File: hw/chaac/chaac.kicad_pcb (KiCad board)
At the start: 2 copper layers, 42 x 55 mm, 56 parts, among them J1 Battery, J2 TC2030-CTX, J3 UART, J4 windrain, Q1 Q_PMOS_GSD, SW1 RST, SW2 RST, U1 TPS7A0530PDBVT, U2 NRF52811-QFAA, U3 BMP280, U4 SHT3x-DIS, U5 E22-X00M22S, Y2 32.768kHz

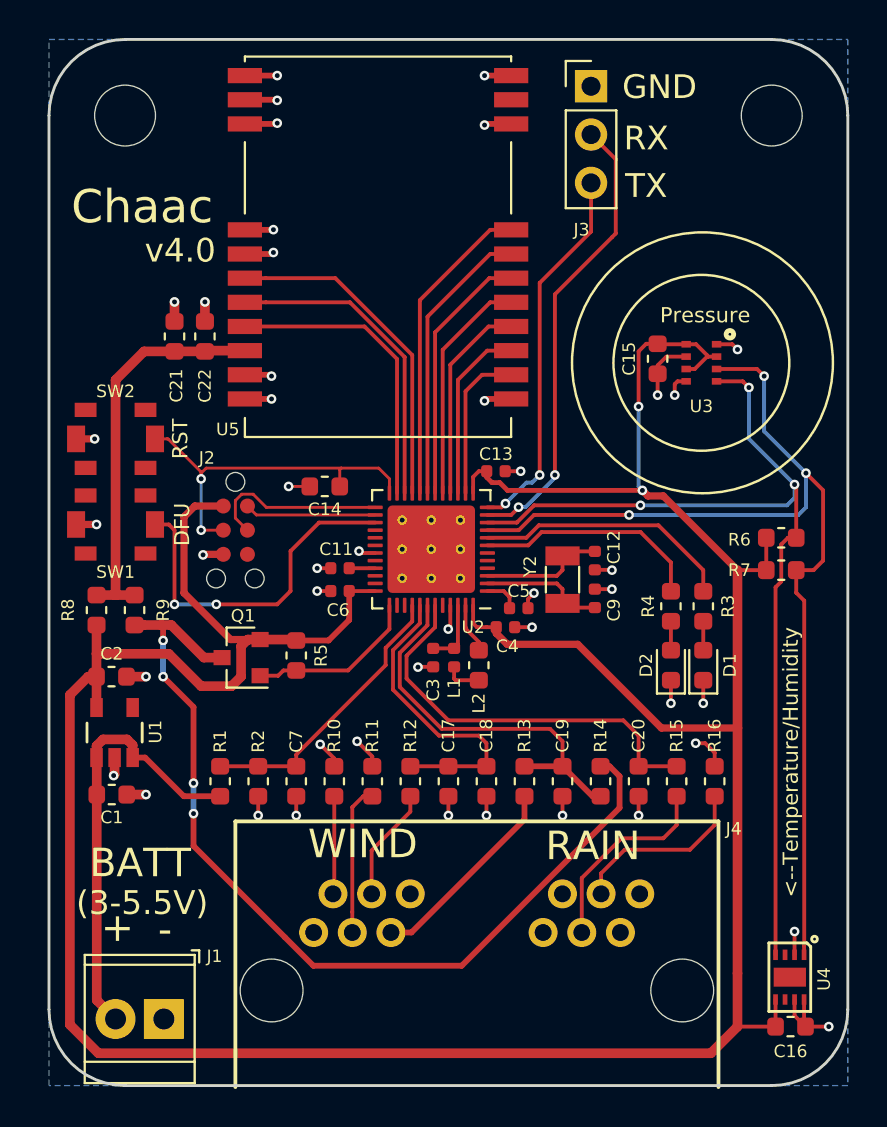
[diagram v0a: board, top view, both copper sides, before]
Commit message: Adding chaac v5.0
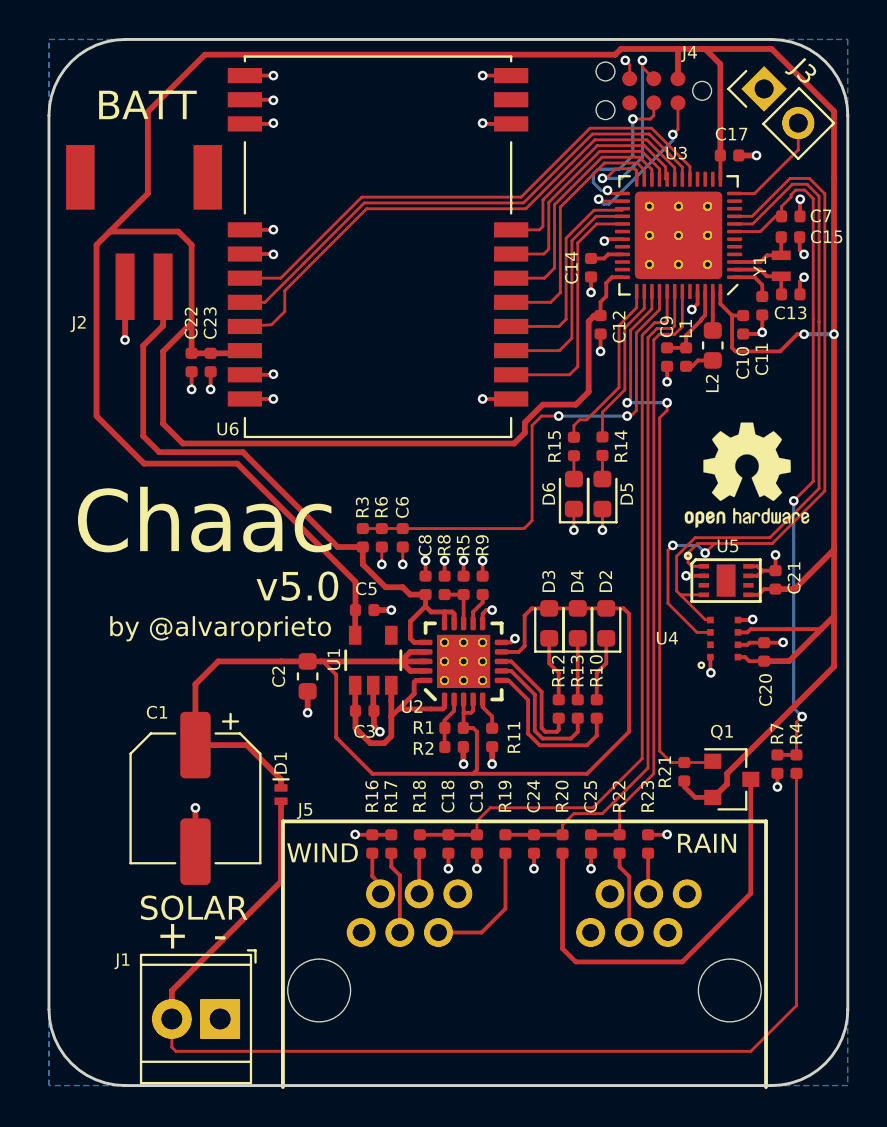
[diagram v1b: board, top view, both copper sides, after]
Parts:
- removed the C14 at (117.5, 152.5)
- removed C16: 0.1uF, Capacitor_SMD:C_0603_1608Metric
- removed the R14 at (132.0, 168.0)
- removed the REF** at (124.4, 151.0)
- removed the REF** at (141.0, 133.0)
- removed the REF** at (107.0, 133.0)
- removed SW1, SW2: RST, alvarop:PTS820J25MSMTRLFS
- removed the U3 at (137.3, 146.0)
- added C2: 10uF, Resistor_SMD:R_0603_1608Metric, F.Cu at (116.6, 162.5)
- added C21: 0.1uF, Capacitor_SMD:C_0402_1005Metric, F.Cu at (141.2, 157.4)
- added C3: 4.7uF, Capacitor_SMD:C_0402_1005Metric, F.Cu at (119.6, 164.3)
- added C7: 0.1uF, Capacitor_SMD:C_0402_1005Metric, F.Cu at (142.0, 138.3)
- added C8: 4.7uF, Capacitor_SMD:C_0402_1005Metric, F.Cu at (122.8, 157.7)
- added D1: RB521CS30L,315, alvarop:RB521CS30L, F.Cu at (115.2, 168.7)
- added D2: LED_ALT, LED_SMD:LED_0603_1608Metric, F.Cu at (132.3, 159.7)
- added D3: LED_ALT, LED_SMD:LED_0603_1608Metric, F.Cu at (129.3, 159.7)
- added D4: LED_ALT, LED_SMD:LED_0603_1608Metric, F.Cu at (130.8, 159.7)
- added G***: LOGO, alvarop:weather_station, B.Cu at (115.0, 156.0)
- added J2: Battery, alvarop:S2B-PH-SM4-TB, F.Cu at (108.0, 142.0)
- added R1: 270k, Resistor_SMD:R_0402_1005Metric, F.Cu at (124.3, 165.2)
- added R10: 10k, Resistor_SMD:R_0402_1005Metric, F.Cu at (131.8, 164.2)
- added R11: 10k, Resistor_SMD:R_0402_1005Metric, F.Cu at (126.3, 165.7)
- added R12: 10k, Resistor_SMD:R_0402_1005Metric, F.Cu at (129.8, 164.2)
- added R13: 10k, Resistor_SMD:R_0402_1005Metric, F.Cu at (130.8, 164.2)
- added R20: 10k, Resistor_SMD:R_0402_1005Metric, F.Cu at (130.0, 171.3)
- added R4: 1M, Resistor_SMD:R_0402_1005Metric, F.Cu at (142.3, 167.1)
- added R5: 100k, Resistor_SMD:R_0402_1005Metric, F.Cu at (124.8, 157.7)
- added REF**: OSHW-Logo2_7.3x6mm_SilkScreen, Symbol:OSHW-Logo2_7.3x6mm_SilkScreen, F.Cu at (139.7, 151.9)
- added U2: MCP73871, alvarop:MCP73871, F.Cu at (124.8, 161.7)
- added U5: SHT3x-DIS, alvarop:SHT3x, F.Cu at (138.6, 157.4)
- C1: value 1uF -> 100uF; footprint Capacitor_SMD:C_0603_1608Metric -> Capacitor_SMD:CP_Elec_6.3x5.4
- C18: renamed from C17; footprint Capacitor_SMD:C_0603_1608Metric -> Capacitor_SMD:C_0402_1005Metric
- C19: renamed from C18; footprint Capacitor_SMD:C_0603_1608Metric -> Capacitor_SMD:C_0402_1005Metric
- C20: renamed from C15; footprint Capacitor_SMD:C_0603_1608Metric -> Capacitor_SMD:C_0402_1005Metric
- C22: renamed from C21; footprint Capacitor_SMD:C_0603_1608Metric -> Capacitor_SMD:C_0402_1005Metric
- C23: renamed from C22; footprint Capacitor_SMD:C_0603_1608Metric -> Capacitor_SMD:C_0402_1005Metric
- C24: renamed from C19; footprint Capacitor_SMD:C_0603_1608Metric -> Capacitor_SMD:C_0402_1005Metric
- C25: renamed from C20; footprint Capacitor_SMD:C_0603_1608Metric -> Capacitor_SMD:C_0402_1005Metric
- C5: renamed from C2; footprint Capacitor_SMD:C_0603_1608Metric -> Capacitor_SMD:C_0402_1005Metric
- C6: renamed from C7; footprint Capacitor_SMD:C_0603_1608Metric -> Capacitor_SMD:C_0402_1005Metric
- J1: value Battery -> Solar
- J3: footprint Connector_PinHeader_2.54mm:PinHeader_1x03_P2.54mm_Vertical -> Connector_PinHeader_2.54mm:PinHeader_1x02_P2.54mm_Vertical
- R14: renamed from R3; footprint Resistor_SMD:R_0603_1608Metric -> Resistor_SMD:R_0402_1005Metric
- R15: renamed from R4; footprint Resistor_SMD:R_0603_1608Metric -> Resistor_SMD:R_0402_1005Metric
- R16: renamed from R10; value 1k -> 0; footprint Resistor_SMD:R_0603_1608Metric -> Resistor_SMD:R_0402_1005Metric
- R17: renamed from R11; footprint Resistor_SMD:R_0603_1608Metric -> Resistor_SMD:R_0402_1005Metric
- R18: renamed from R12; footprint Resistor_SMD:R_0603_1608Metric -> Resistor_SMD:R_0402_1005Metric
- R19: renamed from R13; footprint Resistor_SMD:R_0603_1608Metric -> Resistor_SMD:R_0402_1005Metric
- R2: footprint Resistor_SMD:R_0603_1608Metric -> Resistor_SMD:R_0402_1005Metric
- R21: renamed from R5; footprint Resistor_SMD:R_0603_1608Metric -> Resistor_SMD:R_0402_1005Metric
- R22: renamed from R15; footprint Resistor_SMD:R_0603_1608Metric -> Resistor_SMD:R_0402_1005Metric
- R23: renamed from R16; footprint Resistor_SMD:R_0603_1608Metric -> Resistor_SMD:R_0402_1005Metric
- R3: renamed from R1; value 100k -> 1M; footprint Resistor_SMD:R_0603_1608Metric -> Resistor_SMD:R_0402_1005Metric
- R6, R7: value 4.7k -> 1M; footprint Resistor_SMD:R_0603_1608Metric -> Resistor_SMD:R_0402_1005Metric
- R8: value 0 -> 100k; footprint Resistor_SMD:R_0603_1608Metric -> Resistor_SMD:R_0402_1005Metric
- R9: value 0 -> 1M; footprint Resistor_SMD:R_0603_1608Metric -> Resistor_SMD:R_0402_1005Metric
- U4: value SHT3x-DIS -> DPS368; footprint alvarop:SHT3x -> alvarop:DPS368
- Y1: renamed from Y2; footprint Crystal:Crystal_SMD_3215-2Pin_3.2x1.5mm -> alvarop:ABS05
- moved J4 31.9 mm to (134.8, 131.7), turned to 180 degrees
- moved Q1 26.6 mm to (138.9, 167.9), turned to 0 degrees
- moved R21 21.3 mm to (136.4, 167.5), turned to 270 degrees
- moved U3 21.0 mm to (136.1, 139.3)
- moved R6 21.0 mm to (120.5, 155.2), turned to 90 degrees
- moved L2 20.8 mm to (137.9, 145.1)
- moved C17 20.7 mm to (138.8, 135.1)
- moved C14 20.6 mm to (131.5, 141.0), turned to 270 degrees
- moved C11 20.4 mm to (140.5, 143.0), turned to 90 degrees
- moved C10 20.2 mm to (139.5, 144.0), turned to 90 degrees
- moved Y1 20.1 mm to (141.5, 140.9), turned to 90 degrees
- moved C9 20.0 mm to (135.5, 145.7)
- moved L1 20.0 mm to (136.5, 145.7)
- moved C15 19.9 mm to (142.0, 139.4), turned to 0 degrees
- moved C12 19.6 mm to (132.0, 144.0), turned to 90 degrees
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- renumbered C4 to C10, C5 to C11, C6 to C12, C9 to C13, C11 to C14, C12 to C15, C13 to C17, C3 to C9, D1 to D5, D2 to D6, J2 to J4, J4 to J5, U2 to U3, U5 to U6
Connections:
- C1 pad 1: /VBATT -> /MCP_VIN
- C22 pad 1: Net-(C21-Pad1) -> +3V3
- C23 pad 1: Net-(C21-Pad1) -> +3V3
- J1 pad 2: /VBATT -> /SOLAR_IN
- J3 pad 2: /UART_RX -> /UART_TX
- R2 pad 1: GND -> Net-(R1-Pad2)
- R2 pad 2: /BATT -> GND
- R6 pad 1: /SCL -> GND
- R6 pad 2: +3V3 -> /BATT
- R7 pad 1: /SDA -> GND
- R7 pad 2: +3V3 -> /VSOLAR
- R8 pad 1: Net-(C21-Pad1) -> GND
- R8 pad 2: +3V3 -> Net-(R5-Pad2)
- R9 pad 1: Net-(C21-Pad1) -> GND
- R9 pad 2: /SNS_3V3 -> Net-(R9-Pad2)
- U1 pad 1: /VBATT -> /VIN
- U1 pad 3: /VBATT -> /VIN
- U3 pad 10: /SCL -> Net-(U3-Pad10)
- U3 pad 11: /UART_RX -> Net-(U3-Pad11)
- U3 pad 14: /E22_DIO1 -> Net-(U3-Pad14)
- U3 pad 15: /E22_BUSY -> Net-(U3-Pad15)
- U3 pad 16: /E22_NRST -> Net-(U3-Pad16)
- U3 pad 17: /MISO -> /E22_RXEN
- U3 pad 18: /MOSI -> /E22_TXEN
- U3 pad 19: /SCK -> /E22_DIO2
- U3 pad 21: /E22_RXEN -> /SCK
- U3 pad 22: /E22_TXEN -> /MOSI
- U3 pad 23: /E22_DIO2 -> /MISO
- U3 pad 27: /BOOT -> /E22_NRST
- U3 pad 28: Net-(U2-Pad28) -> /E22_BUSY
- U3 pad 29: Net-(U2-Pad29) -> /E22_DIO1
- U3 pad 37: /SNS_3V3_EN -> /LED2
- U3 pad 38: Net-(U2-Pad38) -> /LED1
- U3 pad 39: Net-(U2-Pad39) -> /SNS_3V3_EN
- U3 pad 7: /LED2 -> /VSOLAR
- U3 pad 8: /LED1 -> /SCL
- U4 pad 1: /SDA -> GND
- U4 pad 2: GND -> Net-(U4-Pad2)
- U4 pad 3: Net-(U4-Pad3) -> /SDA
- U4 pad 5: +3V3 -> GND
- U4 pad 6: Net-(U4-Pad6) -> +3V3
- U4 pad 8: GND -> +3V3
- U6 pad 9: Net-(C21-Pad1) -> +3V3
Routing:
- net /MCP_VIN: track 0.00 -> 66.8 mm
- net /SOLAR_IN: track 0.00 -> 61.5 mm
- net /VSOLAR: track 0.00 -> 36.6 mm, vias 0 -> 2
- net +3V3: track 169.0 -> 202.0 mm
- net /SNS_3V3: track 48.9 -> 22.7 mm, vias 4 -> 0
- net /UART_RX: track 24.3 -> 0.00 mm, vias 2 -> 0
- net /WSPEED: track 16.3 -> 39.2 mm
- net /SNS_3V3_EN: track 9.06 -> 30.0 mm, vias 0 -> 2
- net Net-(C21-Pad1): track 20.7 -> 0.00 mm
- net /BOOT: track 18.6 -> 0.00 mm, vias 2 -> 0
- net /SCL: track 50.6 -> 35.4 mm, vias 3 -> 0
- net /WDIR: track 20.6 -> 35.4 mm
- net /SDA: track 54.5 -> 40.2 mm, vias 3 -> 2
- net /UART_TX: track 19.9 -> 5.71 mm, vias 2 -> 0
- net /VIN: track 0.00 -> 13.2 mm
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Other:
- board text added: "4B"
- board text added: "SOLAR"
- board text added: "https://github.com/alvarop/chaac"
- board text added: "v5.0"
- board text removed: "(3-5.5V)"
- board text removed: "<--Temperature/Humidity"
- board text removed: "DFU"
- board text removed: "GND"
- board text removed: "Pressure"
- board text removed: "RST"
- board text removed: "RX"
- board text removed: "TX"
- board text removed: "https://github.com/alvarop/chaac/"
- board text removed: "v4.0"
